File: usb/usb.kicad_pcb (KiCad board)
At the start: 2 copper layers, 55 x 40 mm, 21 parts, among them J1 USB_B, J2 SPI, J3 C2 interface, J4 UART, J5 TWI, J6 GPIO1, J7 GPIO2, J8 GPIO3, U1 C8051F320

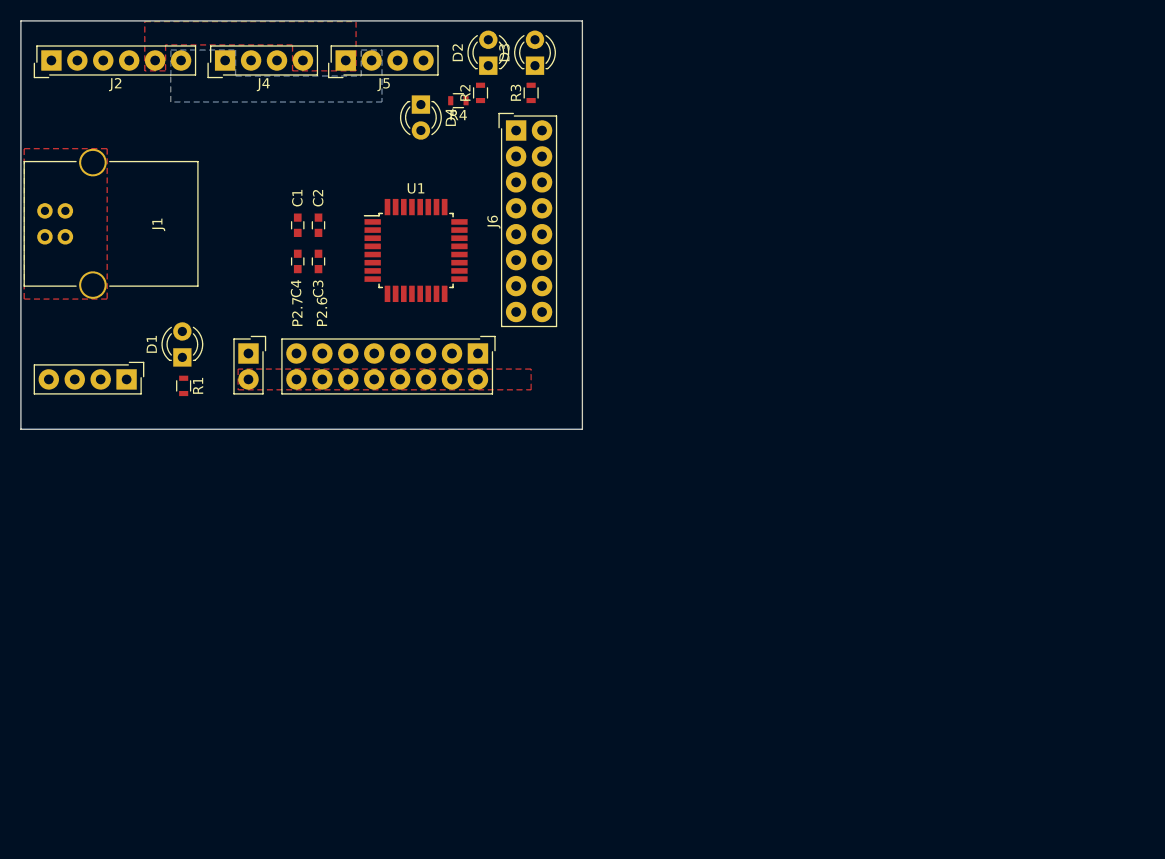
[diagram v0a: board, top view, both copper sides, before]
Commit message: improve usb board
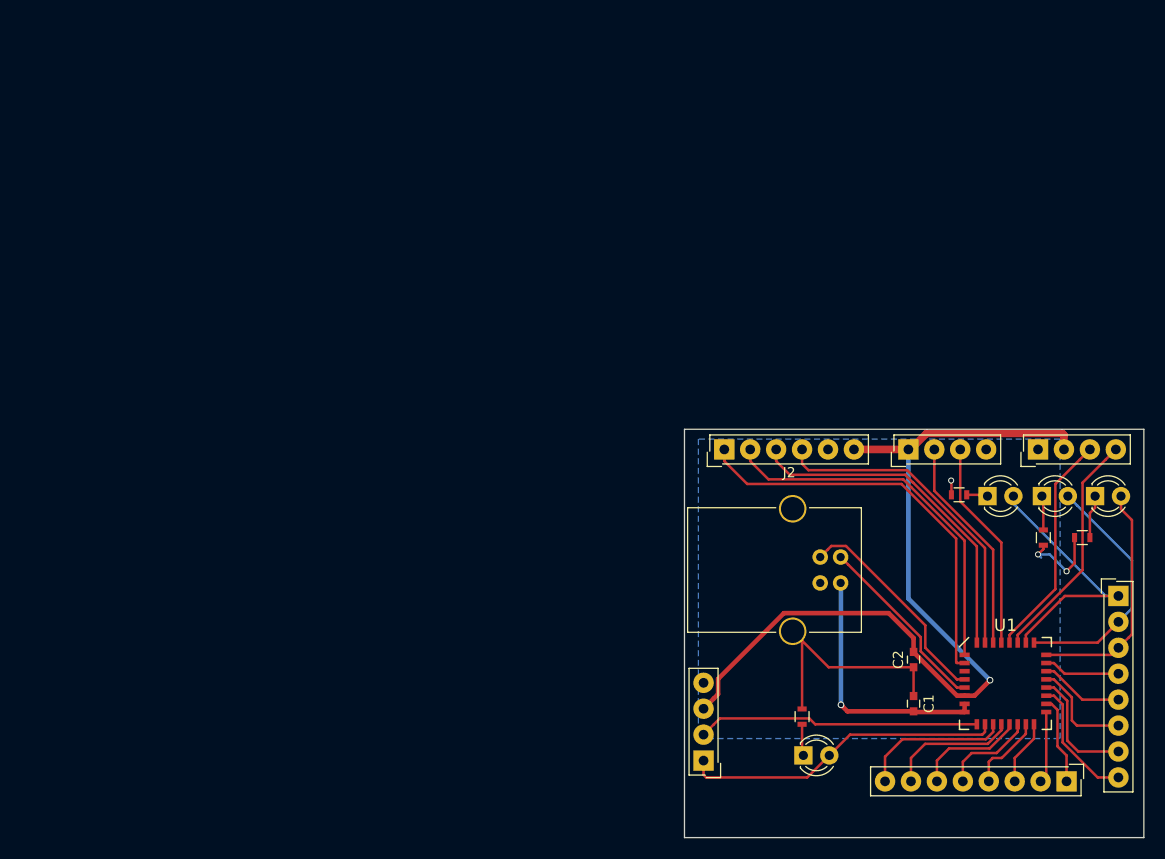
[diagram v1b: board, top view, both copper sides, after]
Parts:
- removed C3: 0.1uF, Capacitors_SMD:C_0603
- removed C4: 4.7uF, Capacitors_SMD:C_0603
- removed J8: GPIO3, Connectors_Samtec:SDL-102-X-XX_2x01
- C1: value 0.1uF -> 4.7uF
- J6, J7: footprint Connectors_Samtec:SDL-116-X-XX_2x08 -> Connectors_Samtec:SL-108-X-XX_1x08
- U1: footprint Housings_QFP:TQFP-32_7x7mm_Pitch0.8mm -> my_footprint:LQFP_32
- moved J1 86.0 mm to (100.3, 75.1), turned to 180 degrees
- moved J5 77.8 mm to (119.6, 62.0)
- moved J4 77.0 mm to (106.9, 62.0)
- moved C1 76.4 mm to (107.4, 86.9)
- moved J2 76.1 mm to (88.9, 62.0)
- moved J6 74.6 mm to (127.5, 76.3)
- moved R2 73.3 mm to (124.0, 70.6), turned to 0 degrees
- moved D2 72.9 mm to (125.2, 66.5), turned to 0 degrees
- moved D1 72.3 mm to (96.6, 91.9), turned to 0 degrees
- moved C2 72.2 mm to (107.4, 82.6), turned to 90 degrees
- moved U1 71.6 mm to (116.4, 84.9)
- moved J7 71.3 mm to (122.4, 94.5)
- moved R1 68.7 mm to (96.5, 88.2), turned to 90 degrees
- moved J3 67.7 mm to (86.9, 92.5), turned to 180 degrees
- moved D4 67.5 mm to (114.7, 66.5), turned to 0 degrees
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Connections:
- net Net-(D1-Pad2) renamed /C2D
- net Net-(J3-Pad2) renamed /C2CK
- net Net-(J4-Pad2) renamed /TXD
- net Net-(J4-Pad3) renamed /RXD
- C1 pad 2: +3V3 -> /Vbus
- J6 pad 2: GND -> Net-(D3-Pad2)
- J6 pad 3: Net-(D3-Pad2) -> Net-(D2-Pad2)
- J6 pad 4: GND -> Net-(J6-Pad4)
- J6 pad 5: Net-(D2-Pad2) -> Net-(J6-Pad5)
- J6 pad 6: GND -> Net-(J6-Pad6)
- J6 pad 8: GND -> Net-(J6-Pad8)
- J7 pad 2: GND -> Net-(J7-Pad2)
- J7 pad 4: GND -> Net-(J7-Pad4)
- J7 pad 6: GND -> Net-(J7-Pad6)
- J7 pad 8: GND -> Net-(J7-Pad8)
- U1 pad 11: Net-(J7-Pad15) -> Net-(J7-Pad8)
- U1 pad 12: Net-(J7-Pad13) -> Net-(J7-Pad7)
- U1 pad 13: Net-(J7-Pad11) -> Net-(J7-Pad6)
- U1 pad 14: Net-(J7-Pad9) -> Net-(J7-Pad5)
- U1 pad 15: Net-(J7-Pad7) -> Net-(J7-Pad4)
- U1 pad 16: Net-(J7-Pad5) -> Net-(J7-Pad3)
- U1 pad 17: Net-(J7-Pad3) -> Net-(J7-Pad2)
- U1 pad 19: Net-(J6-Pad15) -> Net-(J6-Pad8)
- U1 pad 20: Net-(J6-Pad13) -> Net-(J6-Pad7)
- U1 pad 21: Net-(J6-Pad11) -> Net-(J6-Pad6)
- U1 pad 22: Net-(J6-Pad9) -> Net-(J6-Pad5)
- U1 pad 23: Net-(J6-Pad7) -> Net-(J6-Pad4)
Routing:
- net +3V3: track 0.00 -> 86.2 mm, vias 0 -> 1
- net Net-(J2-Pad1): track 0.00 -> 40.0 mm
- net Net-(J2-Pad2): track 0.00 -> 36.6 mm
- net GND: track 0.00 -> 34.2 mm, vias 0 -> 3
- net Net-(J2-Pad3): track 0.00 -> 33.7 mm
- net Net-(J2-Pad4): track 0.00 -> 32.0 mm
- net /C2D: track 0.00 -> 31.7 mm
- net /C2CK: track 0.00 -> 27.7 mm
- net Net-(D4-Pad2): track 0.00 -> 26.2 mm
- net /Vbus: track 0.00 -> 25.2 mm, vias 0 -> 1
- net Net-(D3-Pad2): track 0.00 -> 24.6 mm
- net Net-(D2-Pad2): track 0.00 -> 23.2 mm
- net Net-(J5-Pad4): track 0.00 -> 22.9 mm
- net Net-(J5-Pad3): track 0.00 -> 22.2 mm
- net /TXD: track 0.00 -> 21.3 mm
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- added copper zone on B.Cu, net GND
- removed copper zone on B.Cu, net +3V3
- removed copper zone on F.Cu, net GND
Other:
- board size 55 x 40 mm -> 45 x 40 mm
- board text removed: "P2.6"
- board text removed: "P2.7"
